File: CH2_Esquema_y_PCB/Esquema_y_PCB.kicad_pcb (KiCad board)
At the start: 2 copper layers, 143.4 x 79.8 mm, 44 parts, among them Q1 BC547, Q10 BC857, Q2 BC547, Q3 BC547, Q4 BC547, Q5 IRF9Z34N, Q7 BC547, Q9 BC857, U1 TL431LP, U2 LM358

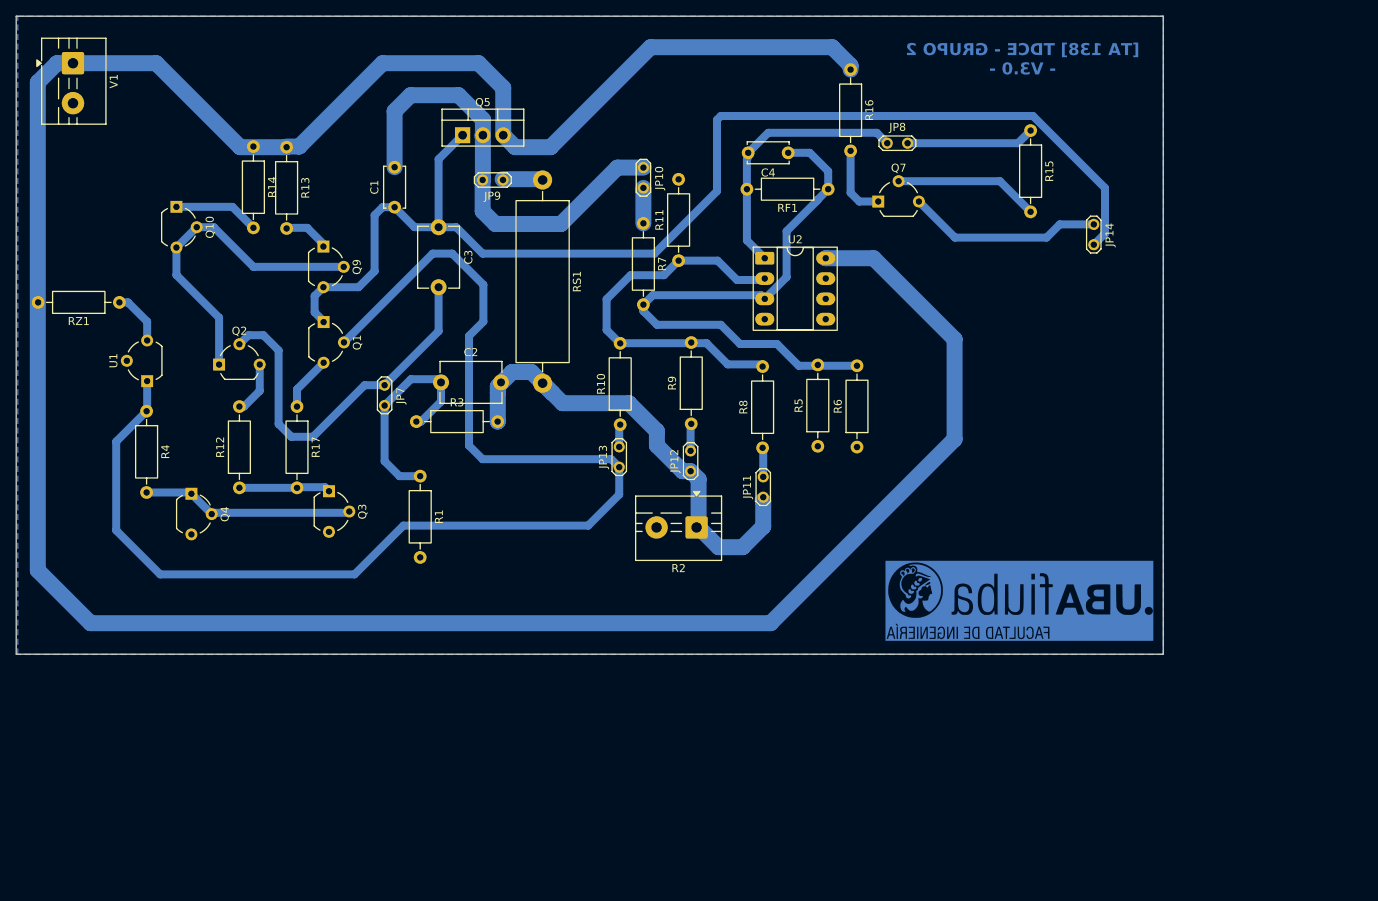
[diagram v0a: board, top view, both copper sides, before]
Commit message: Add files via upload
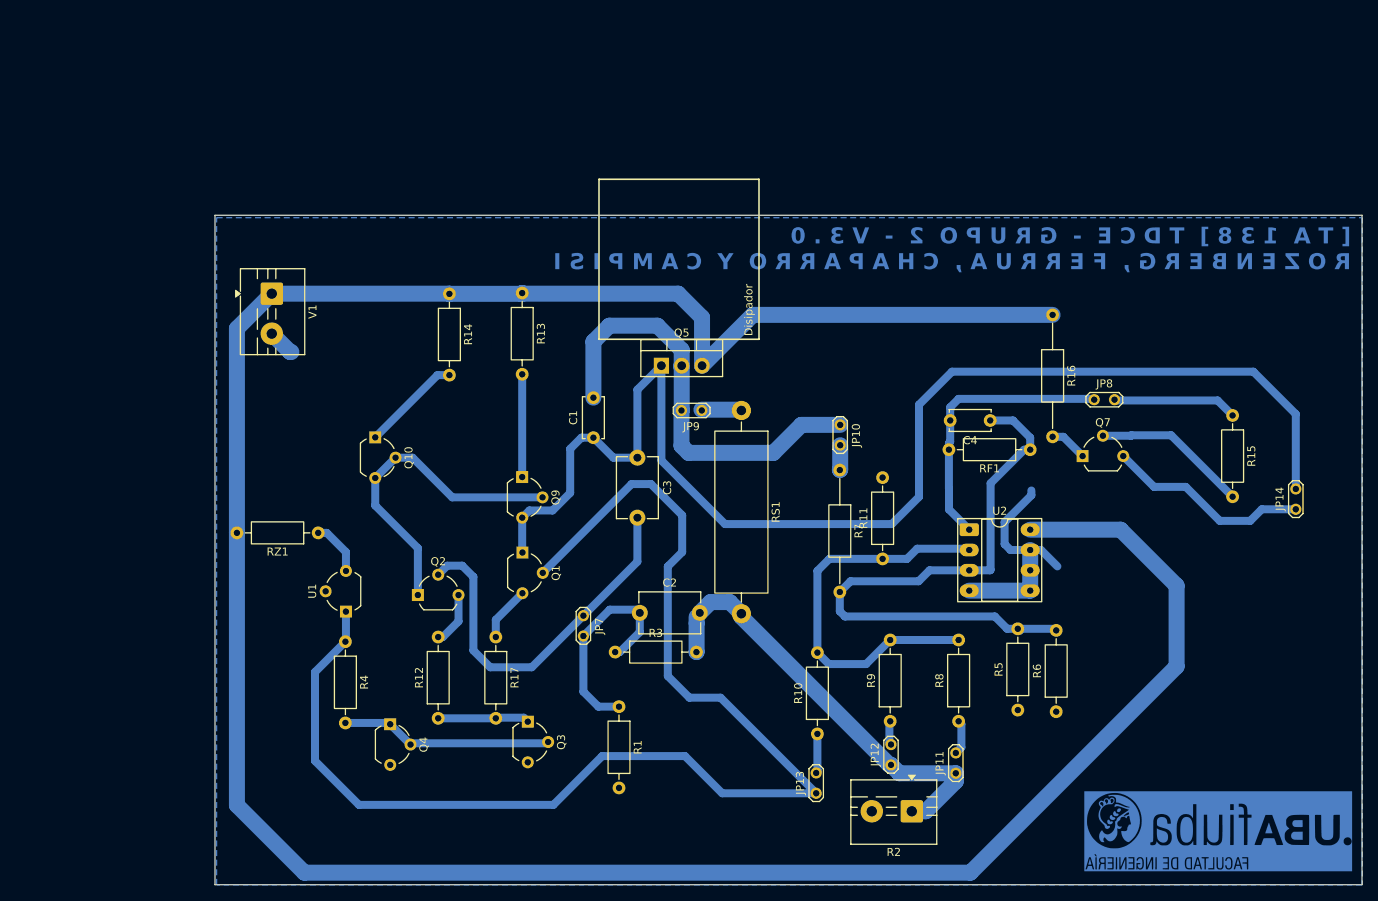
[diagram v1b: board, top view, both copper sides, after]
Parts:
- R16, R7: footprint Resistor_THT:R_Axial_DIN0207_L6.3mm_D2.5mm_P10.16mm_Horizontal -> Resistor_THT:R_Axial_DIN0207_L6.3mm_D2.5mm_P15.24mm_Horizontal
- moved JP13 47.6 mm to (143.7, 132.3)
- moved R10 45.8 mm to (143.8, 124.8)
- moved R11 45.2 mm to (152.0, 103.0)
- moved R9 44.7 mm to (152.9, 123.3)
- moved R2 44.5 mm to (155.7, 134.5)
- moved JP12 44.4 mm to (153.1, 128.7)
- moved JP14 43.7 mm to (203.7, 96.8), turned to 90 degrees
- moved R15 43.7 mm to (195.8, 85.0)
- moved U2 42.5 mm to (162.8, 99.3)
- moved JP11 42.1 mm to (161.2, 129.8)
- moved R8 42.1 mm to (161.5, 123.3)
- moved C4 41.9 mm to (165.4, 85.7)
- moved R6 41.4 mm to (173.7, 122.1)
- moved R5 41.4 mm to (168.9, 121.9)
- moved RF1 41.2 mm to (170.4, 89.3)
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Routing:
- net GND: track 0.00 -> 31.9 mm
- net VCC: track 346.5 -> 336.4 mm
- net /gate: track 150.2 -> 160.0 mm
- net Net-(Q9-E): track 5.76 -> 12.8 mm
- net Net-(Q7-C): track 9.15 -> 4.75 mm
- net /out: track 59.6 -> 55.2 mm
- net Net-(U2A-+): track 71.7 -> 75.8 mm
- net Net-(JP13-B): track 2.88 -> 5.27 mm
- net Net-(U2A--): track 48.1 -> 49.9 mm
- net Net-(JP8-A): track 33.1 -> 34.9 mm
- net Net-(Q10-E): track 10.9 -> 12.5 mm
- net /drain: track 55.4 -> 53.9 mm
- net /in: track 157.4 -> 158.8 mm
- net Net-(Q7-B): track 18.1 -> 19.4 mm
- net Net-(JP10-B): track 4.43 -> 3.13 mm
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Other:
- board size 143.4 x 79.8 mm -> 143.4 x 83.7 mm
- board text added: "Disipador"
- board text added: "[ T A 1 3 8 ] T D C E - G R U P O 2 - V 3 . 0 R O Z E N B E R G , F E R R U A , C H A P A R R O Y C A M P I S I"
- board text removed: "[TA 138] TDCE - GRUPO 2 - V3.0 -"
